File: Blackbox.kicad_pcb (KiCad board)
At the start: 4 copper layers, 77 x 34.5 mm, 38 parts, among them CN1 SM04B-SRSS-TB (LF)(SN), U1 SN65HVD232DR, U2 STM32G0B1CCT6, U3 BM06B-SRSS-TB(LF)(SN), X2 DSX321G-48M

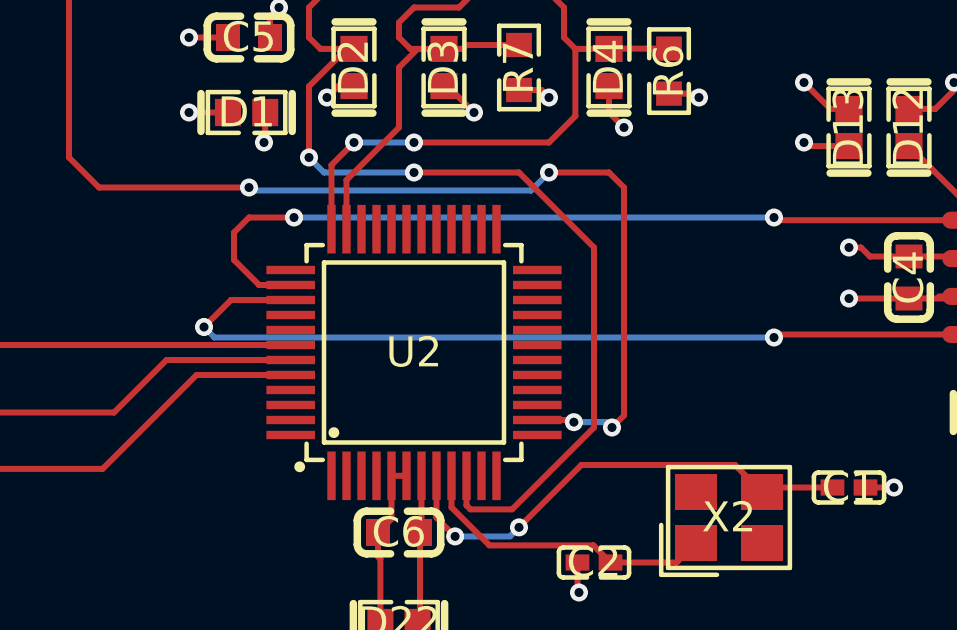
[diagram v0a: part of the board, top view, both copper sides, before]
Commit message: PCB update
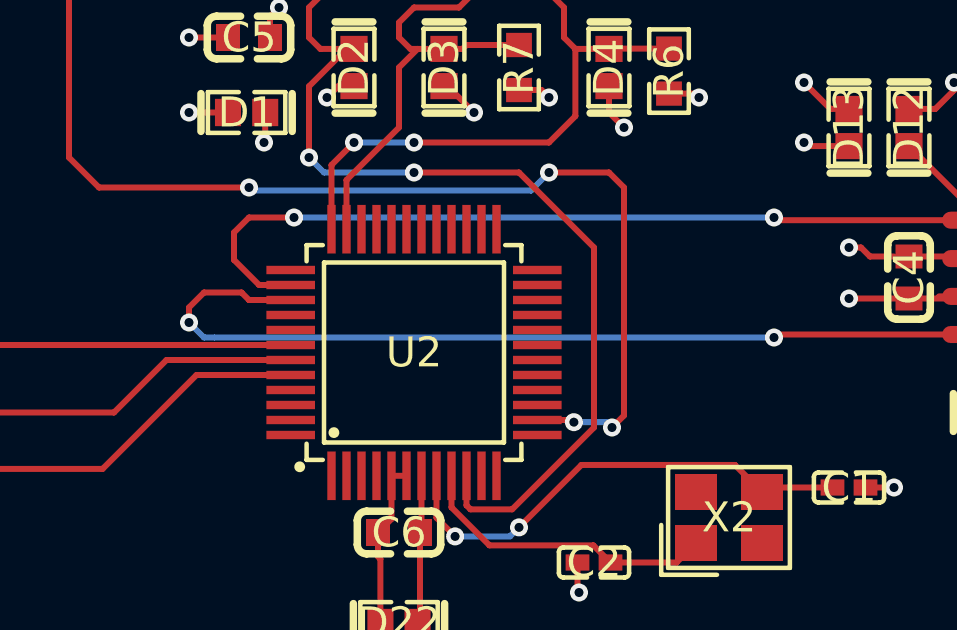
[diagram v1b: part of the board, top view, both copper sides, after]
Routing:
- net RX: track 31.8 -> 33.3 mm
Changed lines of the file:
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@@
+	)
+	(segment
+		(start 136.5 104)
+		(end 136.5 103.5)
+		(width 0.2)
+		(layer "F.Cu")
+		(net 23)
+	)
+	(segment
+		(start 136.5 103.5)
+		(end 137 103)
+		(width 0.2)
+		(layer "F.Cu")
+		(net 23)
 	)
 	(segment
 		(start 162.88 104.7)
 		(end 162.58 104.4)
+		(width 0.2)
+		(layer "F.Cu")
+		(net 23)
+	)
+	(segment
+		(start 137 103)
+		(end 138.25 103)
 		(width 0.2)
 		(layer "F.Cu")
@@
 	)
 	(segment
-		(start 137 104.15)
-		(end 137.9 103.25)
+		(start 138.25 103)
+		(end 138.5 103.25)
 		(width 0.2)
 		(layer "F.Cu")
@@
 	)
 	(segment
-		(start 137.9 103.25)
+		(start 138.5 103.25)
 		(end 139.89 103.25)
 		(width 0.2)
@@
 	)
 	(via
-		(at 137 104.15)
+		(at 136.5 104)
 		(size 0.6)
 		(drill 0.3)
@@
 	(segment
 		(start 137.35 104.5)
-		(end 137 104.15)
+		(end 137 104.5)
 		(width 0.2)
 		(layer "B.Cu")
@@
 	)
 	(segment
-		(start 156 104.5)
-		(end 137.35 104.5)
+		(start 137 104.5)
+		(end 136.5 104)
 		(width 0.2)
 		(layer "B.Cu")
+		(net 23)
+	)
+	(segment
+		(start 137.35 104.5)
+		(end 156 104.5)
+		(width 0.2)
+		(layer "B.Cu")
